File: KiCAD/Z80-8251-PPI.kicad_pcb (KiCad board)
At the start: 2 copper layers, 99.7 x 74.9 mm, 31 parts, among them J1 SBC8080 BUS, J2 8251-CE, J3 PPI-CE, J4 232C-CON, J5 CON-A, J6 CON-B, J7 OPM-CE, P1 Power, P2 Analog, P3 Digital, P4 Digital, P5 CONN_01X01, P6 CONN_01X01, P7 CONN_01X01, P8 CONN_01X01, Q1 2SC1815, U1 74HC138, U2 8251, U3 8255, U4 74HC4060, Y1 4.9152MHz

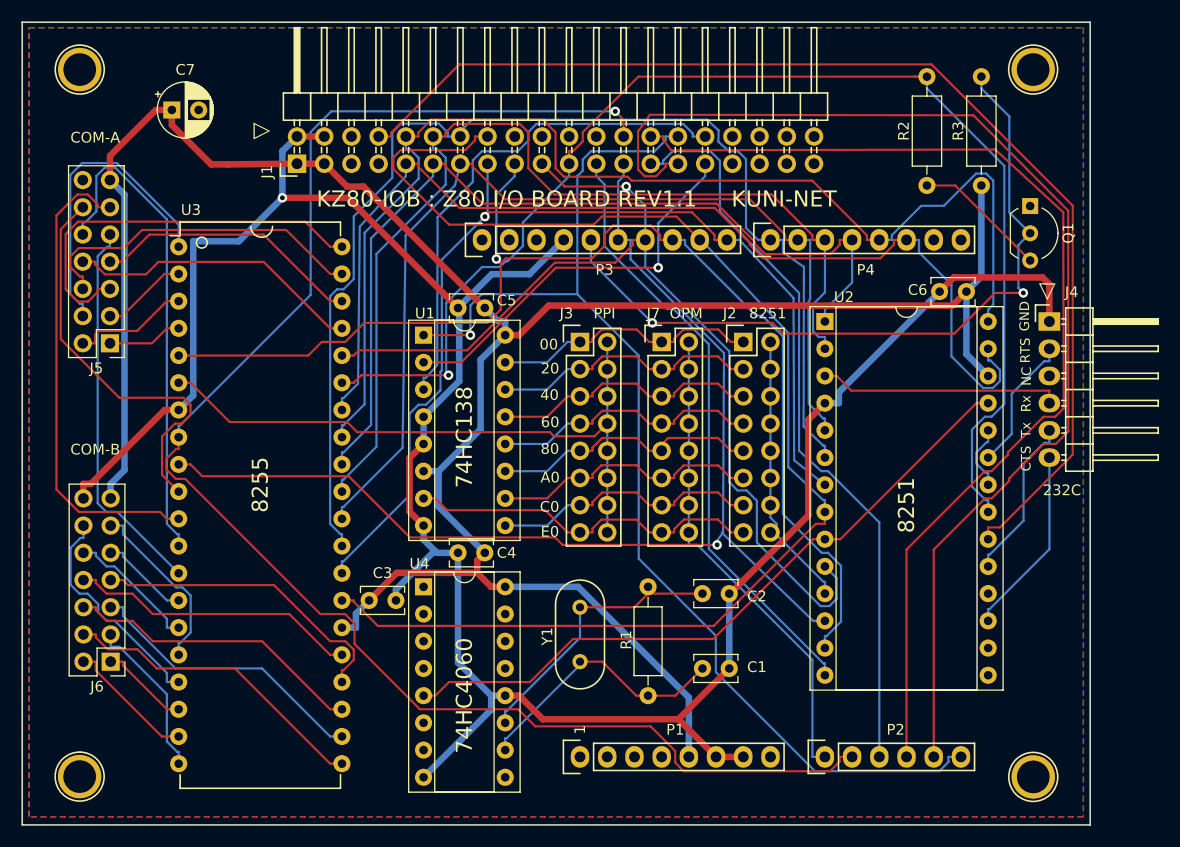
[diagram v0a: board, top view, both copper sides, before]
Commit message: REV2 回路図、製造データ出力
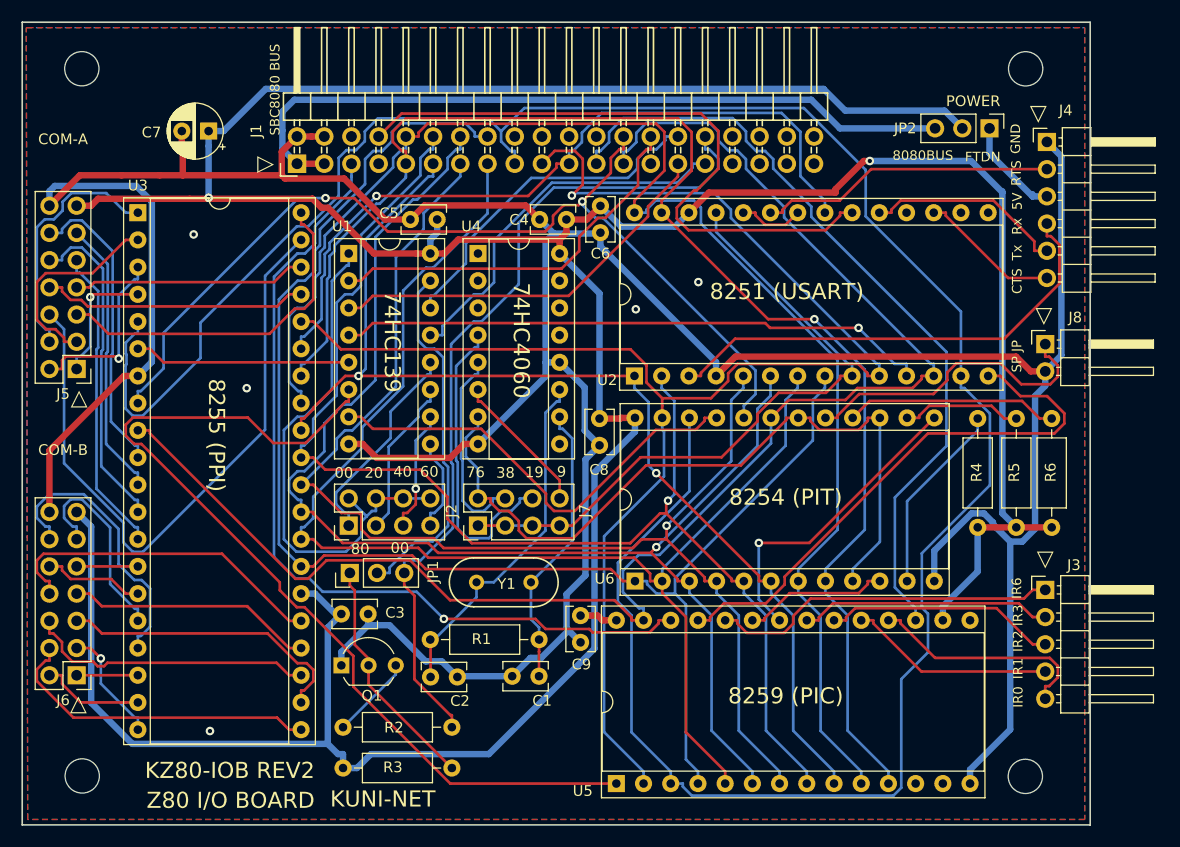
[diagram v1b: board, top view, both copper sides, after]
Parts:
- removed P1: Power, Socket_Arduino_Uno:Socket_Strip_Arduino_1x08
- removed P2: Analog, Socket_Arduino_Uno:Socket_Strip_Arduino_1x06
- removed P3: Digital, Socket_Arduino_Uno:Socket_Strip_Arduino_1x10
- removed P4: Digital, Socket_Arduino_Uno:Socket_Strip_Arduino_1x08
- removed P5, P6, P7, P8: CONN_01X01, Socket_Arduino_Uno:Arduino_1pin
- added C8: 0.1u, Capacitor_THT:C_Rect_L4.0mm_W2.5mm_P2.50mm, F.Cu at (135.0, 99.9)
- added C9: 0.1u, Capacitor_THT:C_Rect_L4.0mm_W2.5mm_P2.50mm, F.Cu at (133.3, 118.3)
- added J8: SP JP, Connector_PinHeader_2.54mm:PinHeader_1x02_P2.54mm_Horizontal, F.Cu at (176.7, 92.9)
- added JP1: A7_JP, Connector_PinHeader_2.54mm:PinHeader_1x03_P2.54mm_Vertical, F.Cu at (111.7, 114.3)
- added JP2: VCC_JP, Connector_PinHeader_2.54mm:PinHeader_1x03_P2.54mm_Vertical, F.Cu at (171.4, 72.8)
- added MH1: MountingHole, MountingHole:MountingHole_3.2mm_M3, F.Cu at (86.7, 67.2)
- added MH2: MountingHole, MountingHole:MountingHole_3.2mm_M3, F.Cu at (174.8, 67.2)
- added MH3: MountingHole, MountingHole:MountingHole_3.2mm_M3, F.Cu at (86.8, 133.2)
- added MH4: MountingHole, MountingHole:MountingHole_3.2mm_M3, F.Cu at (174.8, 133.3)
- added R4: 100k, Resistor_THT:R_Axial_DIN0207_L6.3mm_D2.5mm_P10.16mm_Horizontal, F.Cu at (170.3, 110.0)
- added R5: 100k, Resistor_THT:R_Axial_DIN0207_L6.3mm_D2.5mm_P10.16mm_Horizontal, F.Cu at (174.0, 110.0)
- added R6: 100k, Resistor_THT:R_Axial_DIN0207_L6.3mm_D2.5mm_P10.16mm_Horizontal, F.Cu at (177.3, 110.0)
- added U5: 8259, Package_DIP:DIP-28_W15.24mm_Socket, F.Cu at (136.6, 133.9)
- added U6: 8254, Package_DIP:DIP-24_W15.24mm_Socket, F.Cu at (138.4, 115.0)
- C1, C2, C3, C4, C5, C6: footprint Capacitors_THT:C_Rect_L4.0mm_W2.5mm_P2.50mm -> Capacitor_THT:C_Rect_L4.0mm_W2.5mm_P2.50mm
- J2: value 8251-CE -> ADDR_JP; footprint Pin_Headers:Pin_Header_Straight_2x08 -> Connector_PinHeader_2.54mm:PinHeader_2x04_P2.54mm_Vertical
- J3: value PPI-CE -> IR JP; footprint Pin_Headers:Pin_Header_Straight_2x08 -> Connector_PinHeader_2.54mm:PinHeader_1x05_P2.54mm_Horizontal
- J4: footprint Pin_Headers:Pin_Header_Angled_1x06 -> Connector_PinHeader_2.54mm:PinHeader_1x06_P2.54mm_Horizontal
- J5, J6: footprint Pin_Headers:Pin_Header_Straight_2x07_Pitch2.54mm -> Connector_PinHeader_2.54mm:PinHeader_2x07_P2.54mm_Vertical
- J7: value OPM-CE -> SERIAL JP; footprint Pin_Headers:Pin_Header_Straight_2x08 -> Connector_PinHeader_2.54mm:PinHeader_2x04_P2.54mm_Vertical
- R1: footprint Resistors_THT:R_Axial_DIN0207_L6.3mm_D2.5mm_P10.16mm_Horizontal -> Resistor_THT:R_Axial_DIN0207_L6.3mm_D2.5mm_P10.16mm_Horizontal
- U1: value 74HC138 -> 74LS139; footprint Housings_DIP:DIP-16_W7.62mm_Socket -> Package_DIP:DIP-16_W7.62mm_Socket
- U2: footprint Housings_DIP:DIP-28_W15.24mm_Socket -> Package_DIP:DIP-28_W15.24mm_Socket
- U3: footprint Housings_DIP:DIP-40_W15.24mm -> Package_DIP:DIP-40_W15.24mm_Socket
- Y1: value 4.9152MHz -> 19.6608MHz
- moved Q1 77.3 mm to (110.9, 122.9), turned to 0 degrees
- moved R2 74.4 mm to (111.1, 128.7), turned to 0 degrees
- moved R3 73.5 mm to (121.3, 132.5), turned to 180 degrees
- moved J3 49.2 mm to (176.7, 115.9)
- moved J2 40.6 mm to (111.6, 109.9), turned to 90 degrees
- moved C6 35.1 mm to (135.1, 80.0), turned to 270 degrees
- moved C4 32.0 mm to (132.0, 81.3)
- moved U4 31.5 mm to (123.7, 84.5)
- moved C2 26.5 mm to (119.3, 124.0)
- moved J7 24.2 mm to (123.7, 109.9), turned to 90 degrees
- moved R1 20.9 mm to (119.2, 120.5), turned to 0 degrees
- moved U2 18.5 mm to (138.3, 95.9), turned to 90 degrees
- moved J4 16.8 mm to (176.8, 74.0)
- moved C1 15.3 mm to (129.4, 123.9), turned to 180 degrees
- moved U1 10.3 mm to (111.6, 84.5)
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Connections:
- J1 pad 1: VCC -> SBC5V
- J1 pad 18: (no net) -> Net-(J1-Pad18)
- J1 pad 20: (no net) -> Net-(J1-Pad20)
- J1 pad 22: (no net) -> Net-(J1-Pad22)
- J1 pad 24: (no net) -> Net-(J1-Pad24)
- J1 pad 27: A2 -> Net-(J1-Pad27)
- J1 pad 3: VCC -> SBC5V
- J1 pad 33: (no net) -> Net-(J1-Pad33)
- J1 pad 34: (no net) -> Net-(J1-Pad34)
- J1 pad 35: (no net) -> Net-(J1-Pad35)
- J1 pad 36: (no net) -> Net-(J1-Pad36)
- J1 pad 37: (no net) -> Net-(J1-Pad37)
- J1 pad 38: (no net) -> Net-(J1-Pad38)
- J1 pad 39: (no net) -> Net-(J1-Pad39)
- J1 pad 40: (no net) -> Net-(J1-Pad40)
- J1 pad 5: (no net) -> ~INTA
- J1 pad 6: (no net) -> Net-(J1-Pad6)
- J1 pad 7: (no net) -> Net-(J1-Pad7)
- J2 pad 2: Net-(J2-Pad10) -> Net-(J2-Pad2)
- J2 pad 4: Net-(J2-Pad10) -> Net-(J2-Pad2)
- J2 pad 6: Net-(J2-Pad10) -> Net-(J2-Pad2)
- J2 pad 8: Net-(J2-Pad10) -> Net-(J2-Pad2)
- J3 pad 1: Net-(J2-Pad1) -> /IR6
- J3 pad 2: Net-(J3-Pad10) -> /IR3
- J3 pad 3: Net-(J2-Pad3) -> /IR2
- J3 pad 4: Net-(J3-Pad10) -> /IR1
- J3 pad 5: Net-(J2-Pad5) -> /IR0
- J4 pad 3: (no net) -> Net-(J4-Pad3)
- J7 pad 1: Net-(J2-Pad1) -> Net-(J7-Pad1)
- J7 pad 2: ~CE -> Net-(J7-Pad2)
- J7 pad 3: Net-(J2-Pad3) -> Net-(J7-Pad1)
- J7 pad 4: ~CE -> Net-(J7-Pad4)
- J7 pad 5: Net-(J2-Pad5) -> Net-(J7-Pad1)
- J7 pad 6: ~CE -> Net-(J7-Pad6)
- J7 pad 7: Net-(J2-Pad7) -> Net-(J7-Pad1)
- J7 pad 8: ~CE -> Net-(J7-Pad8)
- Q1 pad 2: /~RESIN -> Net-(JP1-Pad1)
- R2 pad 2: RES -> A7
- R3 pad 1: VCC -> Net-(JP1-Pad1)
- R3 pad 2: /~RESIN -> VCC
- U1 pad 1: A5 -> Net-(J2-Pad2)
- U1 pad 10: Net-(J2-Pad11) -> Net-(J2-Pad5)
- U1 pad 11: Net-(J2-Pad9) -> Net-(J2-Pad3)
- U1 pad 12: Net-(J2-Pad7) -> Net-(J2-Pad1)
- U1 pad 13: Net-(J2-Pad5) -> A6
- U1 pad 14: Net-(J2-Pad3) -> A5
- U1 pad 15: Net-(J2-Pad1) -> Net-(JP1-Pad2)
- U1 pad 2: A6 -> A3
- U1 pad 3: A7 -> A4
- U1 pad 4: GND -> 8251A-CS
- U1 pad 5: GND -> 8255-CS
- U1 pad 6: VCC -> 8259-CS
- U1 pad 7: Net-(J2-Pad15) -> 8254-CS
- U1 pad 9: Net-(J2-Pad13) -> Net-(J2-Pad7)
- U2 pad 11: Net-(J2-Pad10) -> 8251A-CS
- U2 pad 14: INT -> 8251-A
- U2 pad 15: (no net) -> Net-(U2-Pad15)
- U2 pad 16: (no net) -> Net-(U2-Pad16)
- U2 pad 18: (no net) -> Net-(U2-Pad18)
- U2 pad 25: Net-(U2-Pad25) -> Net-(J7-Pad1)
- U2 pad 9: Net-(U2-Pad25) -> Net-(J7-Pad1)
- U3 pad 6: Net-(J3-Pad10) -> 8255-CS
- U4 pad 1: (no net) -> Net-(U4-Pad1)
- U4 pad 13: (no net) -> Net-(U4-Pad13)
- U4 pad 14: (no net) -> Net-(U4-Pad14)
- U4 pad 15: (no net) -> Net-(U4-Pad15)
- U4 pad 2: (no net) -> Net-(U4-Pad2)
- U4 pad 3: (no net) -> Net-(U4-Pad3)
- U4 pad 4: (no net) -> Net-(J7-Pad6)
- U4 pad 5: Net-(U2-Pad25) -> Net-(J7-Pad4)
- U4 pad 6: (no net) -> Net-(J7-Pad8)
- U4 pad 7: (no net) -> Net-(J7-Pad2)
- U4 pad 9: (no net) -> Net-(U4-Pad9)
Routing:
- net VCC: track 219.9 -> 368.0 mm, vias 0 -> 2
- net ~IOR: track 112.0 -> 229.8 mm, vias 1 -> 0
- net GND: track 231.5 -> 334.3 mm, vias 1 -> 5
- net 8259-CS: track 0.00 -> 87.2 mm
- net ~INTA: track 0.00 -> 80.7 mm, vias 0 -> 1
- net A5: track 108.5 -> 32.2 mm, vias 1 -> 0
- net A4: track 110.1 -> 37.6 mm
- net Net-(J7-Pad2): track 0.00 -> 70.9 mm
- net SBC5V: track 0.00 -> 70.5 mm
- net A2: track 69.7 -> 0.00 mm
- net /~RESIN: track 69.5 -> 0.00 mm, vias 2 -> 0
- net Net-(U2-Pad25): track 64.0 -> 0.00 mm
- net A3: track 99.5 -> 36.7 mm
- net Net-(J7-Pad1): track 0.00 -> 62.0 mm
- net Net-(J3-Pad10): track 60.3 -> 0.00 mm
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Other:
- net class BOLD: trace_width 0.6096 -> 0.6; via_dia 0.889 -> 0.8; via_drill 0.635 -> 0.4
- net class Default: trace_width 0.2032 -> 0.25; via_dia 0.889 -> 0.8; via_drill 0.635 -> 0.4
- rule via_min_drill: 0.06096 -> 0.4
- rule via_min_size: 0.889 -> 0.8
- board text added: "19"
- board text added: "38"
- board text added: "5V"
- board text added: "74HC139"
- board text added: "76"
- board text added: "8080BUS"
- board text added: "8251 (USART)"
- board text added: "8254 (PIT)"
- board text added: "8255 (PPI)"
- board text added: "8259 (PIC)"
- board text added: "9"
- board text added: "FTDN"
- board text added: "IR0"
- board text added: "IR1"
- board text added: "IR2"
- board text added: "IR3"
- board text added: "IR6"
- board text added: "KZ80-IOB REV2"
- board text added: "POWER"
- board text added: "SBC8080 BUS"
- board text added: "SP JP"
- board text added: "Z80 I/O BOARD"
- board text removed: "1"
- board text removed: "232C"
- board text removed: "74HC138"
- board text removed: "8251"
- board text removed: "8255"
- board text removed: "A0"
- board text removed: "C0"
- board text removed: "E0"
- board text removed: "KZ80-IOB : Z80 I/O BOARD REV1.1"
- board text removed: "NC"
- board text removed: "OPM"
- board text removed: "PPI"
